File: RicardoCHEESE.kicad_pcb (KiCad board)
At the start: 4 copper layers, 148 parts, among them IC1 SiC437BED-T1-GE3, J1 RBUS, J2 USB_C_Receptacle_USB2.0, J3 Conn_Coaxial, J4 Conn_01x06_Pin, J5 Conn_01x06_Pin, J6 Conn_01x06_Pin, J7 Conn_01x06_Pin, J8 Conn_01x02_Male, U1 ESP32-S3, U2 SN65HVD230, U3 LM66200DRLR, U4 SC4215, U5 MAX77827AEFD+T, U6 SE5005L, U7 RTC6705, U8 HEF4051BT, Y1 40MHz±10ppm, Y2 8MHz

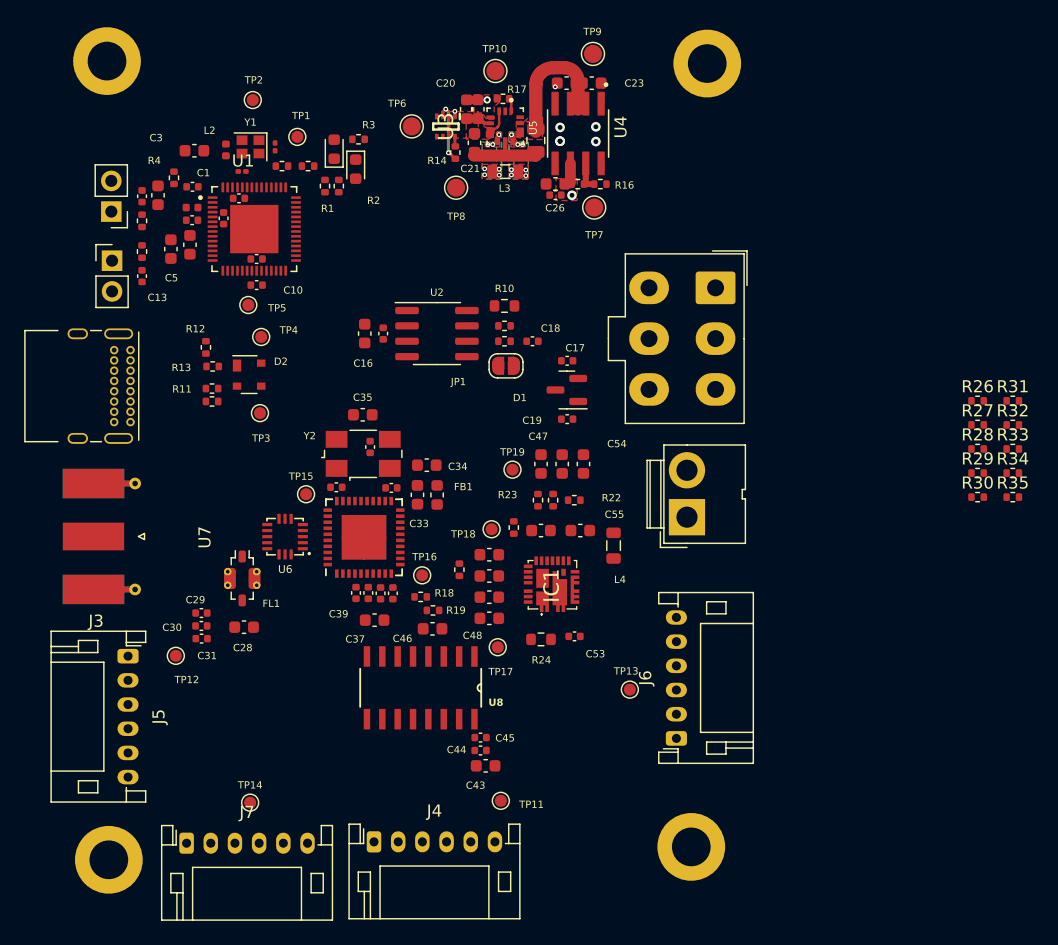
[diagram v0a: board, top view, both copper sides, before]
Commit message: User saved
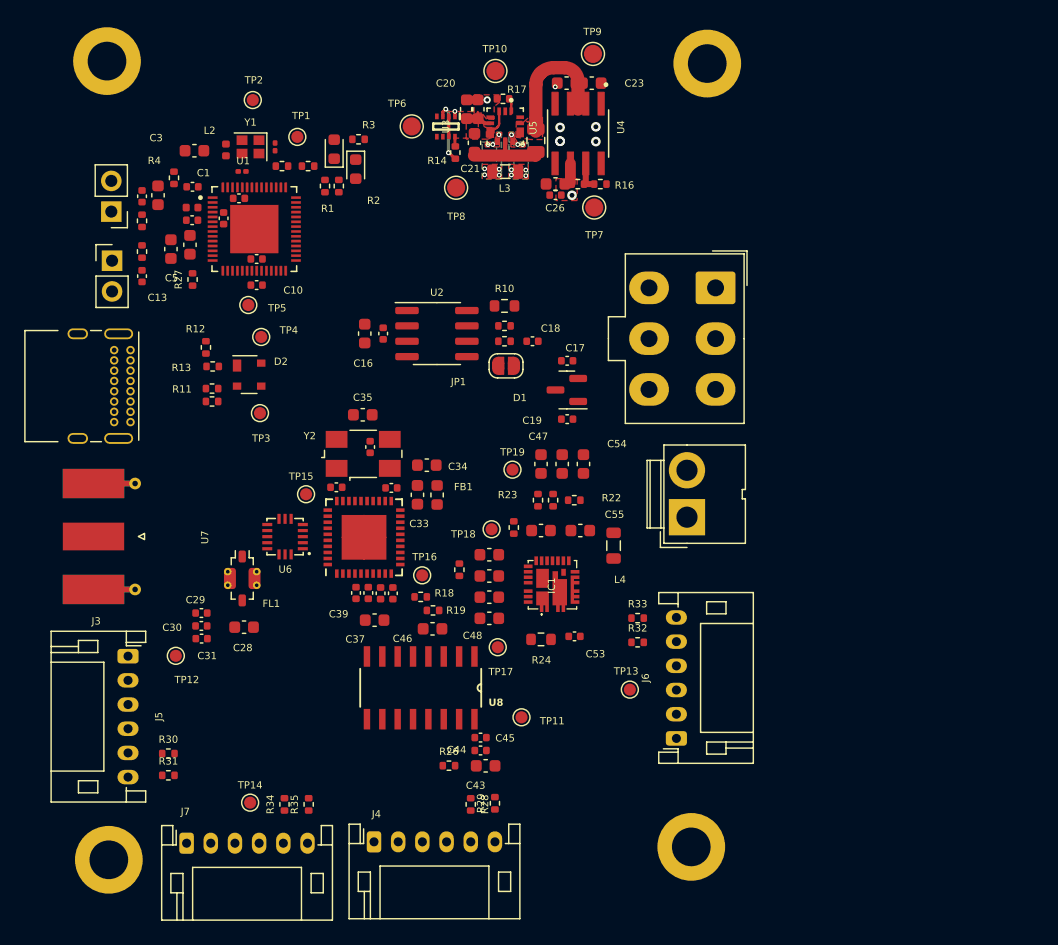
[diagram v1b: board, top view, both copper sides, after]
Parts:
- moved R31 76.4 mm to (142.8, 122.1)
- moved R30 70.2 mm to (142.8, 120.3)
- moved R34 66.2 mm to (152.4, 124.5), turned to 90 degrees
- moved R27 66.0 mm to (144.8, 81.1), turned to 90 degrees
- moved R35 63.5 mm to (154.4, 124.5), turned to 90 degrees
- moved R26 53.1 mm to (166.0, 121.3)
- moved R28 51.2 mm to (167.8, 124.5), turned to -90 degrees
- moved R29 48.4 mm to (169.8, 124.4), turned to 90 degrees
- moved R32 35.9 mm to (181.6, 111.1)
- moved R33 34.0 mm to (181.6, 109.1)
- moved TP11 7.11 mm to (172.0, 117.3)
